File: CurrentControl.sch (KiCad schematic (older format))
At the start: 7 parts

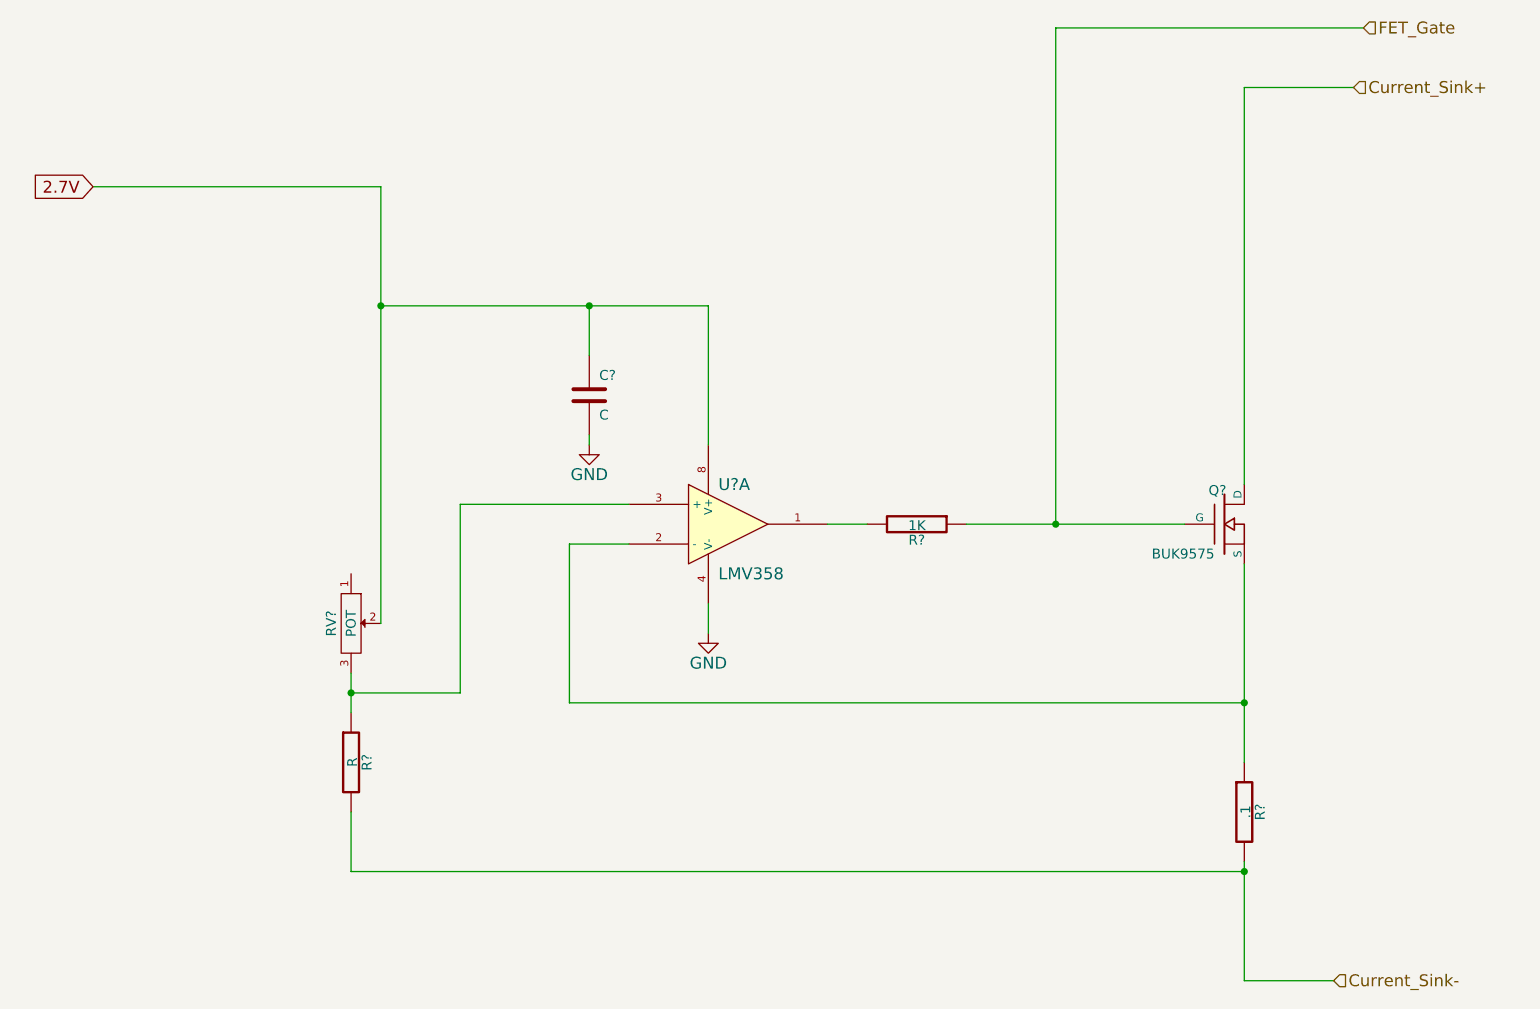
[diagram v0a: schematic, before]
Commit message: Initial Annotation
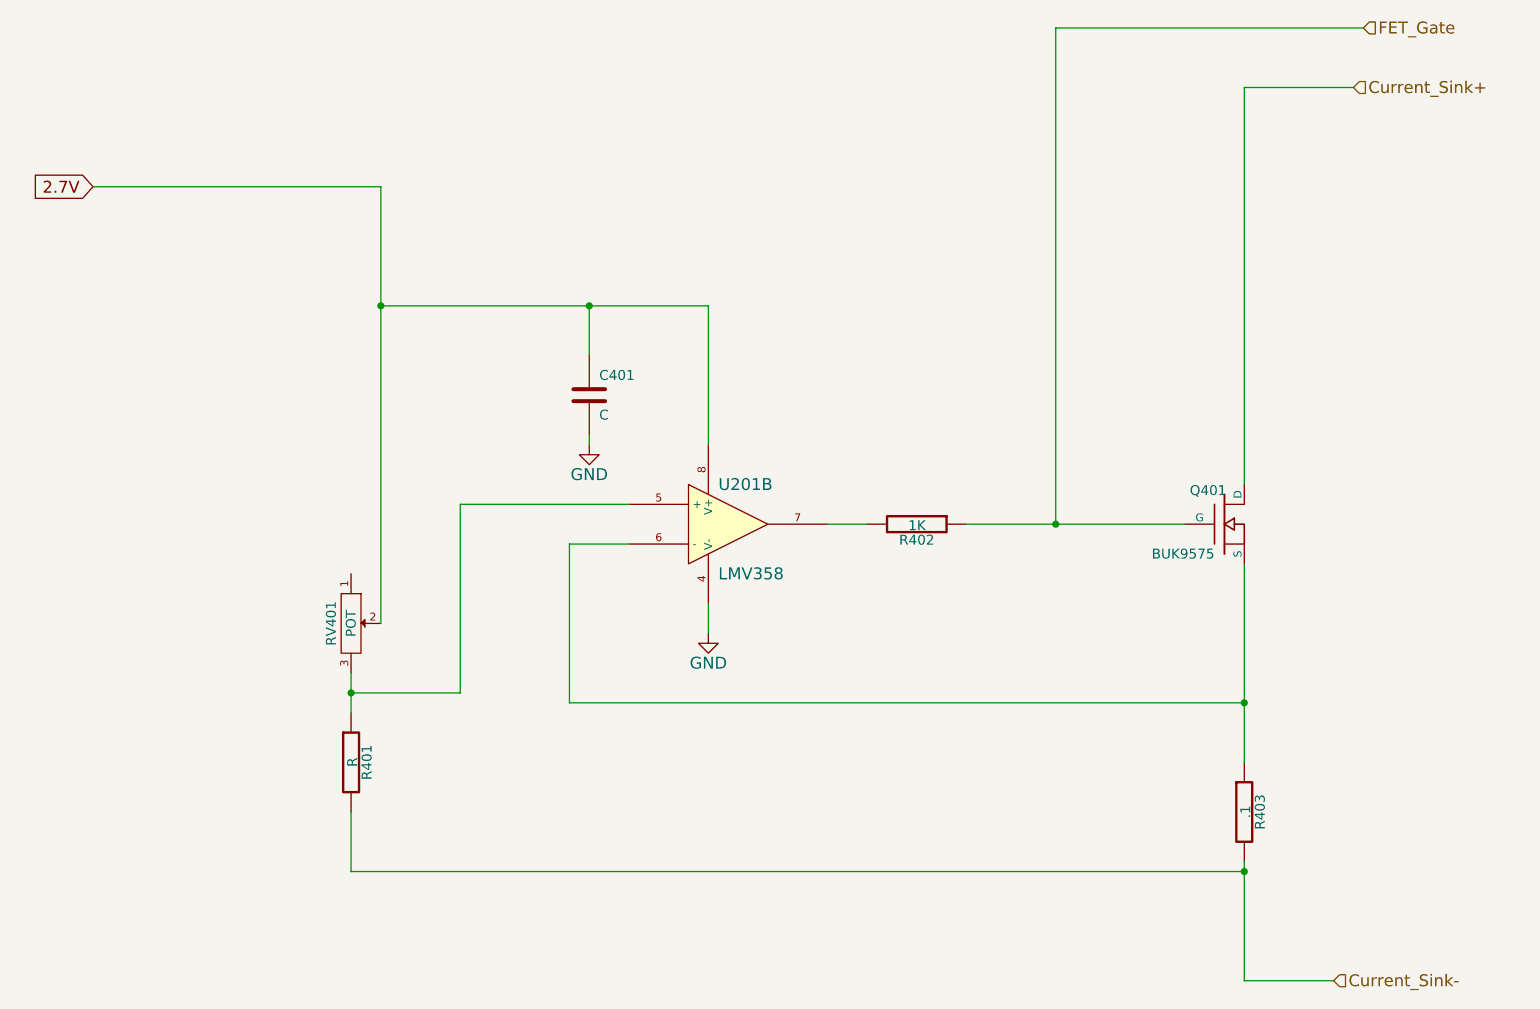
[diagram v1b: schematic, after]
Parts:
- gave numbers to parts that had none: 7
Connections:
- net at R402.2: now also U201.7; no longer U201.1
- net at Q401.S, R403.1: now also U201.6 (-); no longer U201.2 (-)
- net at R401.1, RV401.3: now also U201.5 (+); no longer U201.3 (+)
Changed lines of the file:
@@
 $EndDescr
 $Comp
-L LMV358 U?
-U 1 1 54DADC5E
+L LMV358 U201
+U 2 1 54DADC5E
 P 5500 3700
-F 0 "U?" H 5450 3900 60  0000 L CNN
+F 0 "U201" H 5450 3900 60  0000 L CNN
 F 1 "LMV358" H 5450 3450 60  0000 L CNN
 F 2 "" H 5500 3700 60  0000 C CNN
 F 3 "" H 5500 3700 60  0000 C CNN
-	1    5500 3700
+	2    5500 3700
 	1    0    0    -1
 $EndComp
 $Comp
-L R R?
+L R R403
 U 1 1 54DADC66
 P 8100 5150
-F 0 "R?" V 8180 5150 50  0000 C CNN
+F 0 "R403" V 8180 5150 50  0000 C CNN
 F 1 ".1" V 8107 5151 50  0000 C CNN
 F 2 "" V 8030 5150 30  0000 C CNN
@@
 $EndComp
 $Comp
-L MOSFET_N Q?
+L MOSFET_N Q401
 U 1 1 54DADC74
 P 8000 3700
-F 0 "Q?" H 8010 3870 50  0000 R CNN
+F 0 "Q401" H 8010 3870 50  0000 R CNN
 F 1 "BUK9575" H 7950 3550 50  0000 R CNN
 F 2 "" H 8000 3700 60  0000 C CNN
@@
 $EndComp
 $Comp
-L R R?
+L R R401
 U 1 1 54DADC7B
 P 3600 4900
-F 0 "R?" V 3680 4900 50  0000 C CNN
+F 0 "R401" V 3680 4900 50  0000 C CNN
 F 1 "R" V 3607 4901 50  0000 C CNN
 F 2 "" V 3530 4900 30  0000 C CNN
@@
 $EndComp
 $Comp
-L GND #PWR?
+L GND #PWR402
 U 1 1 54DADC82
 P 5400 4250
-F 0 "#PWR?" H 5400 4000 60  0001 C CNN
+F 0 "#PWR402" H 5400 4000 60  0001 C CNN
 F 1 "GND" H 5400 4100 60  0000 C CNN
 F 2 "" H 5400 4250 60  0000 C CNN
@@
 Connection ~ 8100 5450
 $Comp
-L POT RV?
+L POT RV401
 U 1 1 54DADC9B
 P 3600 4200
-F 0 "RV?" H 3600 4100 50  0000 C CNN
+F 0 "RV401" H 3600 4100 50  0000 C CNN
 F 1 "POT" H 3600 4200 50  0000 C CNN
 F 2 "" H 3600 4200 60  0000 C CNN
@@
 Connection ~ 3750 2600
 $Comp
-L GND #PWR?
+L GND #PWR401
 U 1 1 54DADCA8
 P 4800 3300
-F 0 "#PWR?" H 4800 3050 60  0001 C CNN
+F 0 "#PWR401" H 4800 3050 60  0001 C CNN
 F 1 "GND" H 4800 3150 60  0000 C CNN
 F 2 "" H 4800 3300 60  0000 C CNN
@@
 $EndComp
 $Comp
-L C C?
+L C C401
 U 1 1 54DADCAE
 P 4800 3050
-F 0 "C?" H 4850 3150 50  0000 L CNN
+F 0 "C401" H 4850 3150 50  0000 L CNN
 F 1 "C" H 4850 2950 50  0000 L CNN
 F 2 "" H 4838 2900 30  0000 C CNN
@@
 	8650 1500 8100 1500
 $Comp
-L R R?
+L R R402
 U 1 1 54DAE31B
 P 6450 3700
-F 0 "R?" V 6530 3700 50  0000 C CNN
+F 0 "R402" V 6530 3700 50  0000 C CNN
 F 1 "1K" V 6457 3701 50  0000 C CNN
 F 2 "" V 6380 3700 30  0000 C CNN
